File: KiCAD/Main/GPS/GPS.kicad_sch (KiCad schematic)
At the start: 18 parts, among them IC1 E22-900M22S, U1 MAX-M8Q, U2 PHA-23LN

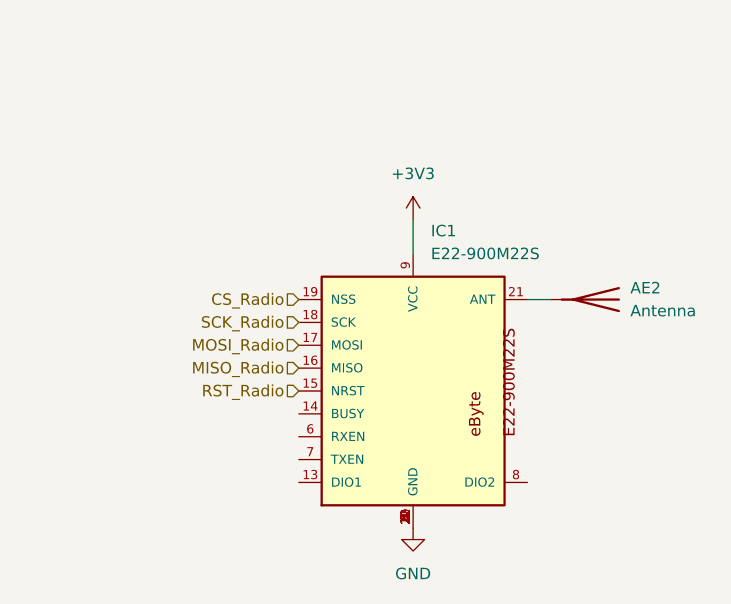
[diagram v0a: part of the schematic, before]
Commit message: Add new rf
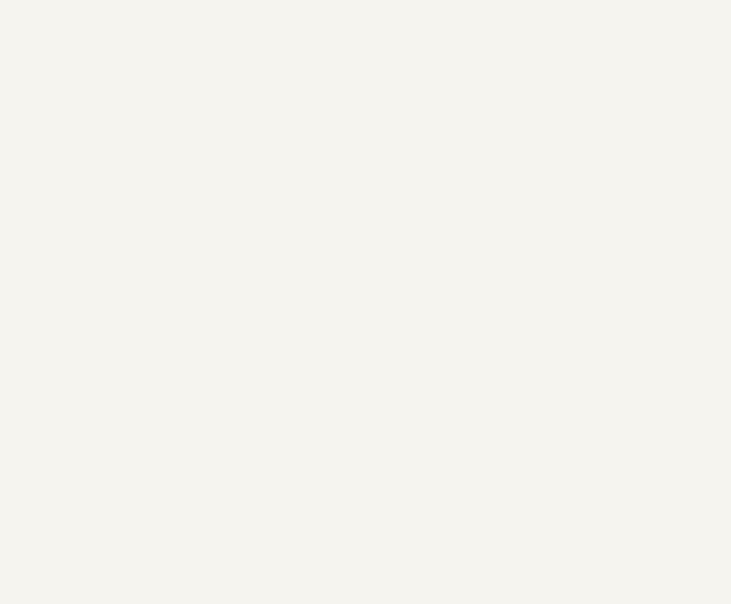
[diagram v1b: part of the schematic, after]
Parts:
- removed AE2: Antenna, symbol Device:Antenna
- removed IC1: E22-900M22S, E22-900M22S:E22-900M22S, symbol E22-900M22S:E22-900M22S
